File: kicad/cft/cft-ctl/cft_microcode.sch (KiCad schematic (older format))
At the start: 15 parts, among them U45 74HC85, U46 74LVC1G00, U47 SN74ACT1071

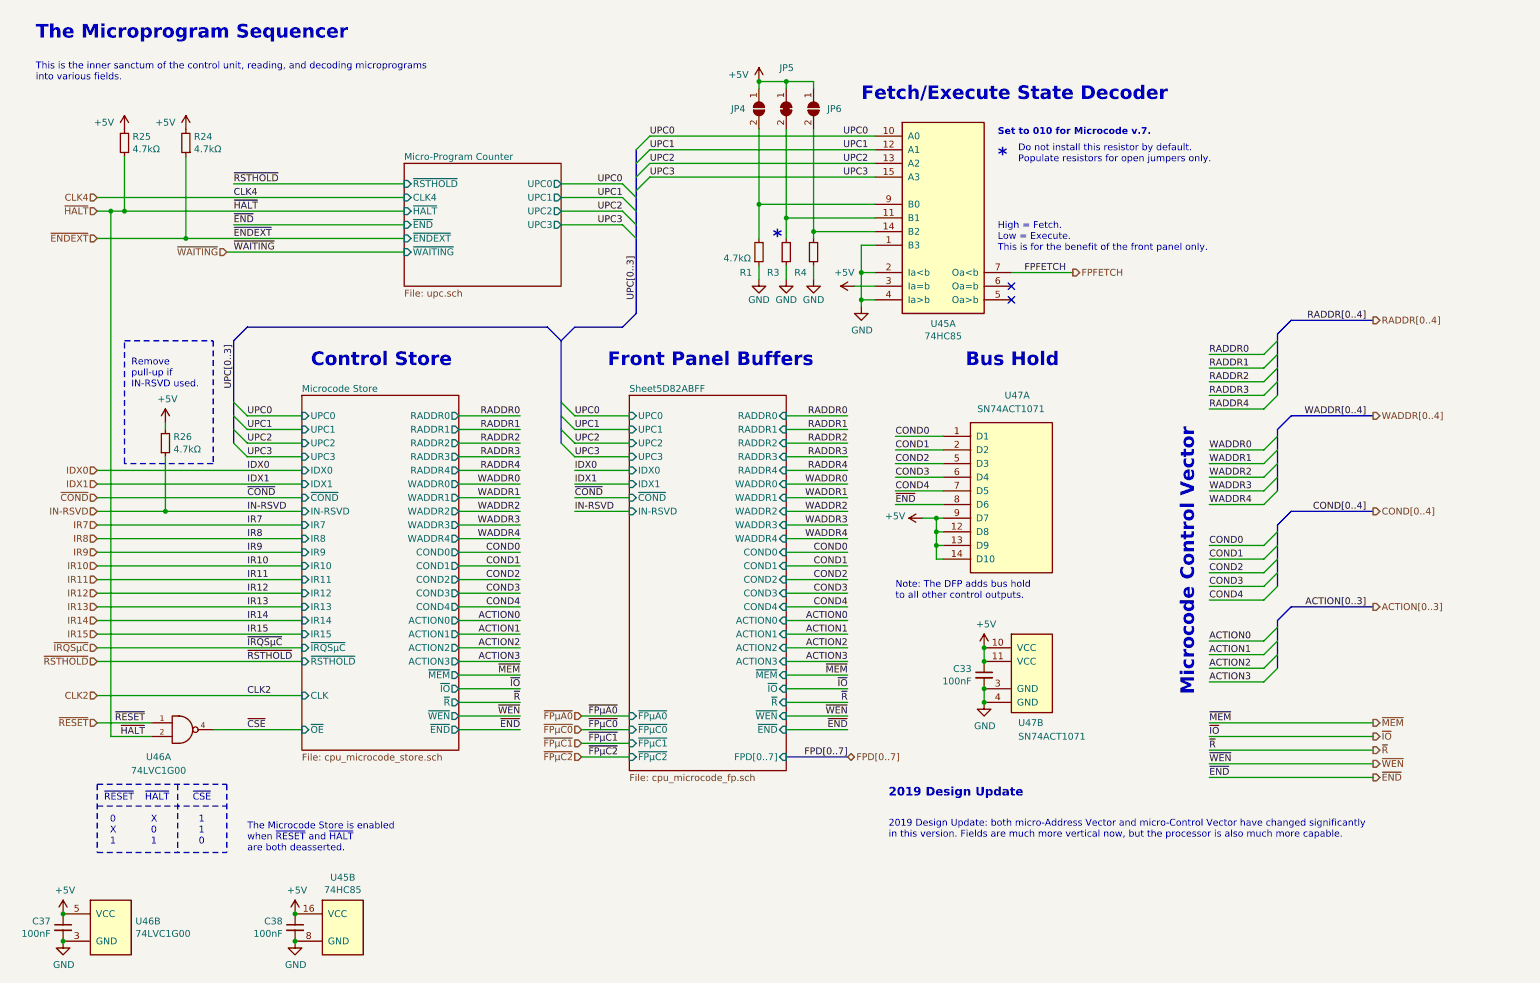
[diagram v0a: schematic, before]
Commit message: Reworking boards for new bus definitions and control store.
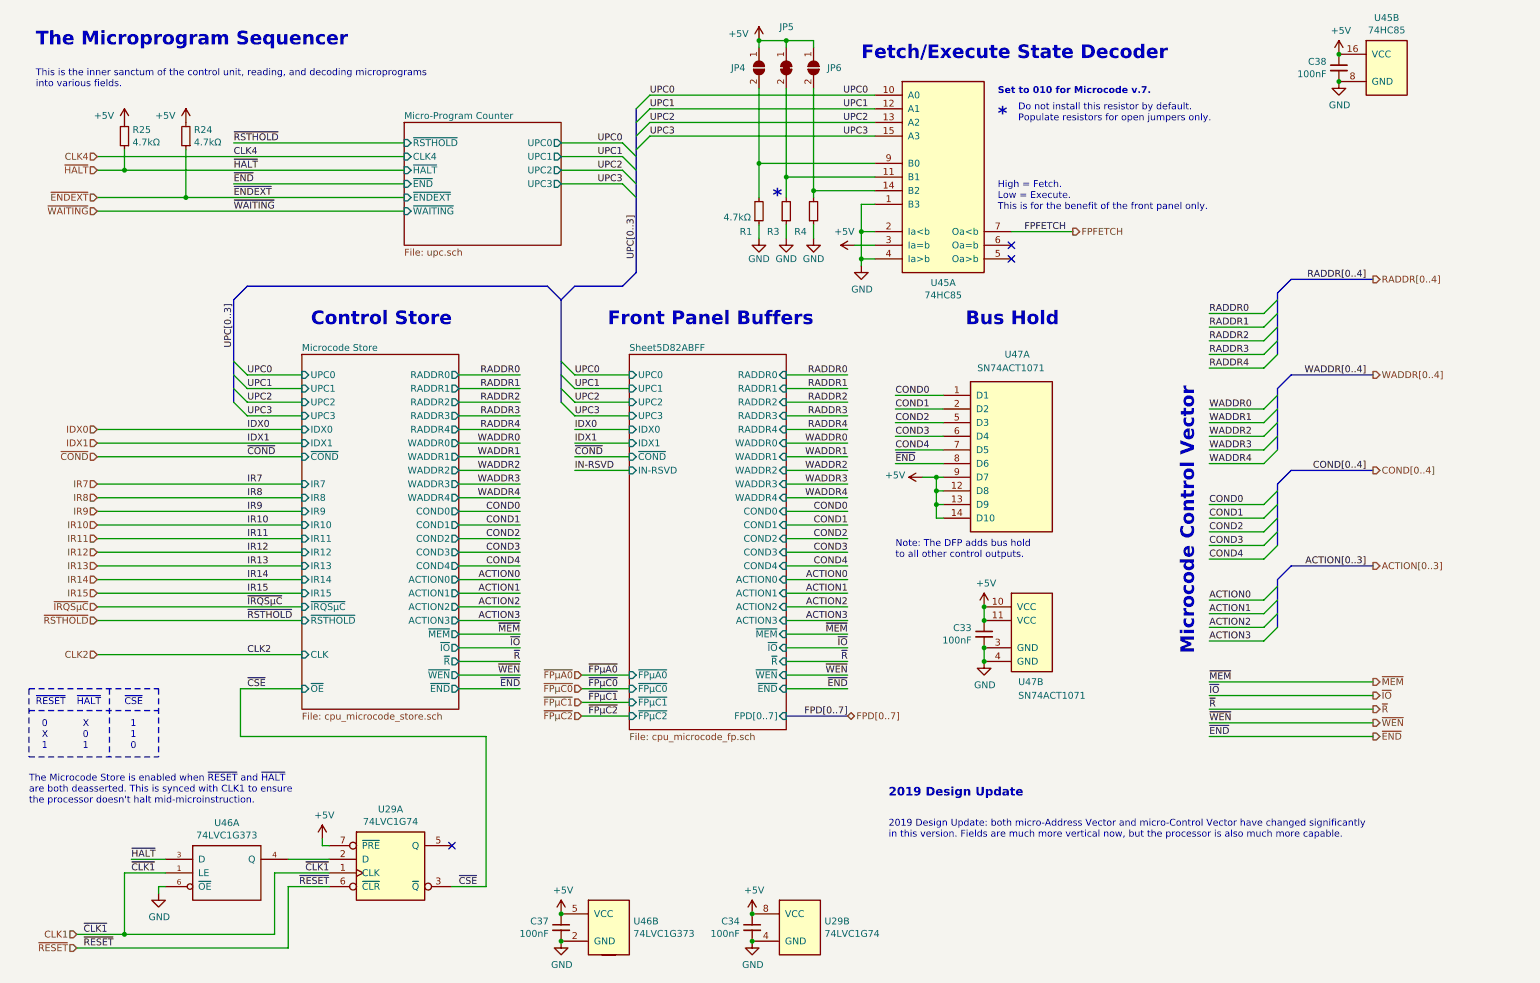
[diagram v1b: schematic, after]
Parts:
- removed R26: 4.7kΩ, alexios:R_SMD_0805_2012Metric_Pad1.15x1.40mm_HandSolder, symbol Device:R_Small
- removed U46: 74LVC1G00, alexios:SOT-23-5_HandSoldering, symbol alexios:74LVC1G00
- added C34: 100nF, alexios:C_SMD_0805_2012Metric_Pad1.15x1.40mm_HandSolder, symbol Device:C_Small
- added U29: 74LVC1G74, alexios:SOIC-8, symbol alexios:74LVC1G74
- added U46: 74LVC1G373, alexios:SOT-23-6_Handsoldering, symbol alexios:74LVC1G373
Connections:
- net +5V: now also C34.1, U29.7 (~PRE), U29.8 (VCC), U46.5 (VCC)
- net GND: now also C34.2, U29.4 (GND), U46.2 (GND), U46.6 (~OE)
- net ~CSE: now also U29.3 (~Q)
- net ~HALT: now also U46.3 (D)
- net ~RESET: now also U29.6 (~CLR)
- new net: U29.2 (D), U46.4 (Q)
- new net CLK1: U29.1 (CLK), U46.1 (LE)
- no-connect marks 2 -> 3
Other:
- note added: "The Microcode Store is enabled when ~RESET~ and ~HALT~\nare both deasserted. This is synced with CLK1 to ensure\nthe processor doesn't halt mid-microinstruction."
- note removed: "Remove\npull-up if\nIN-RSVD used."
- note removed: "The Microcode Store is enabled\nwhen ~RESET~ and ~HALT~\nare both deasserted."
- moved on the sheet: C33, C37, C38, JP4, JP5, JP6, R1, R24, R25, R3, R4, U45A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
